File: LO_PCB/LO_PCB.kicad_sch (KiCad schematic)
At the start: 97 parts, among them J1 PWR, J2 Conn_01x06, Q1 AO3401A, U1 TPS7A9101DSKT, U2 LMX2582RHAR, X1 TB612-100.0M

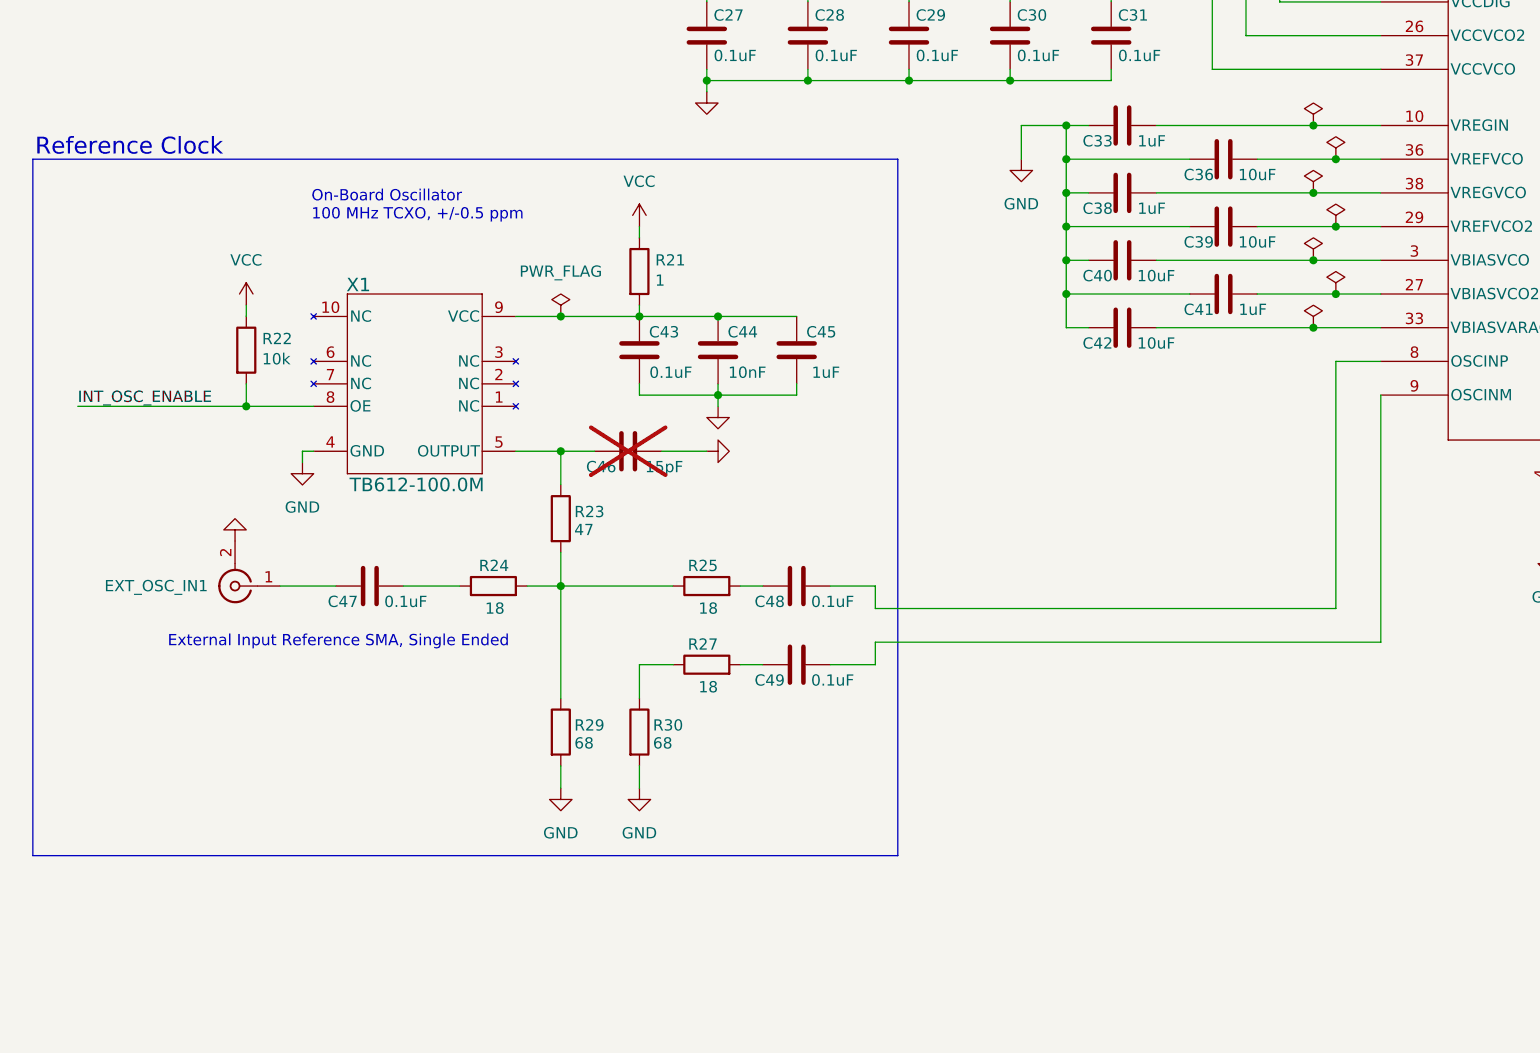
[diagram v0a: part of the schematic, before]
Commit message: final final LO PCB?
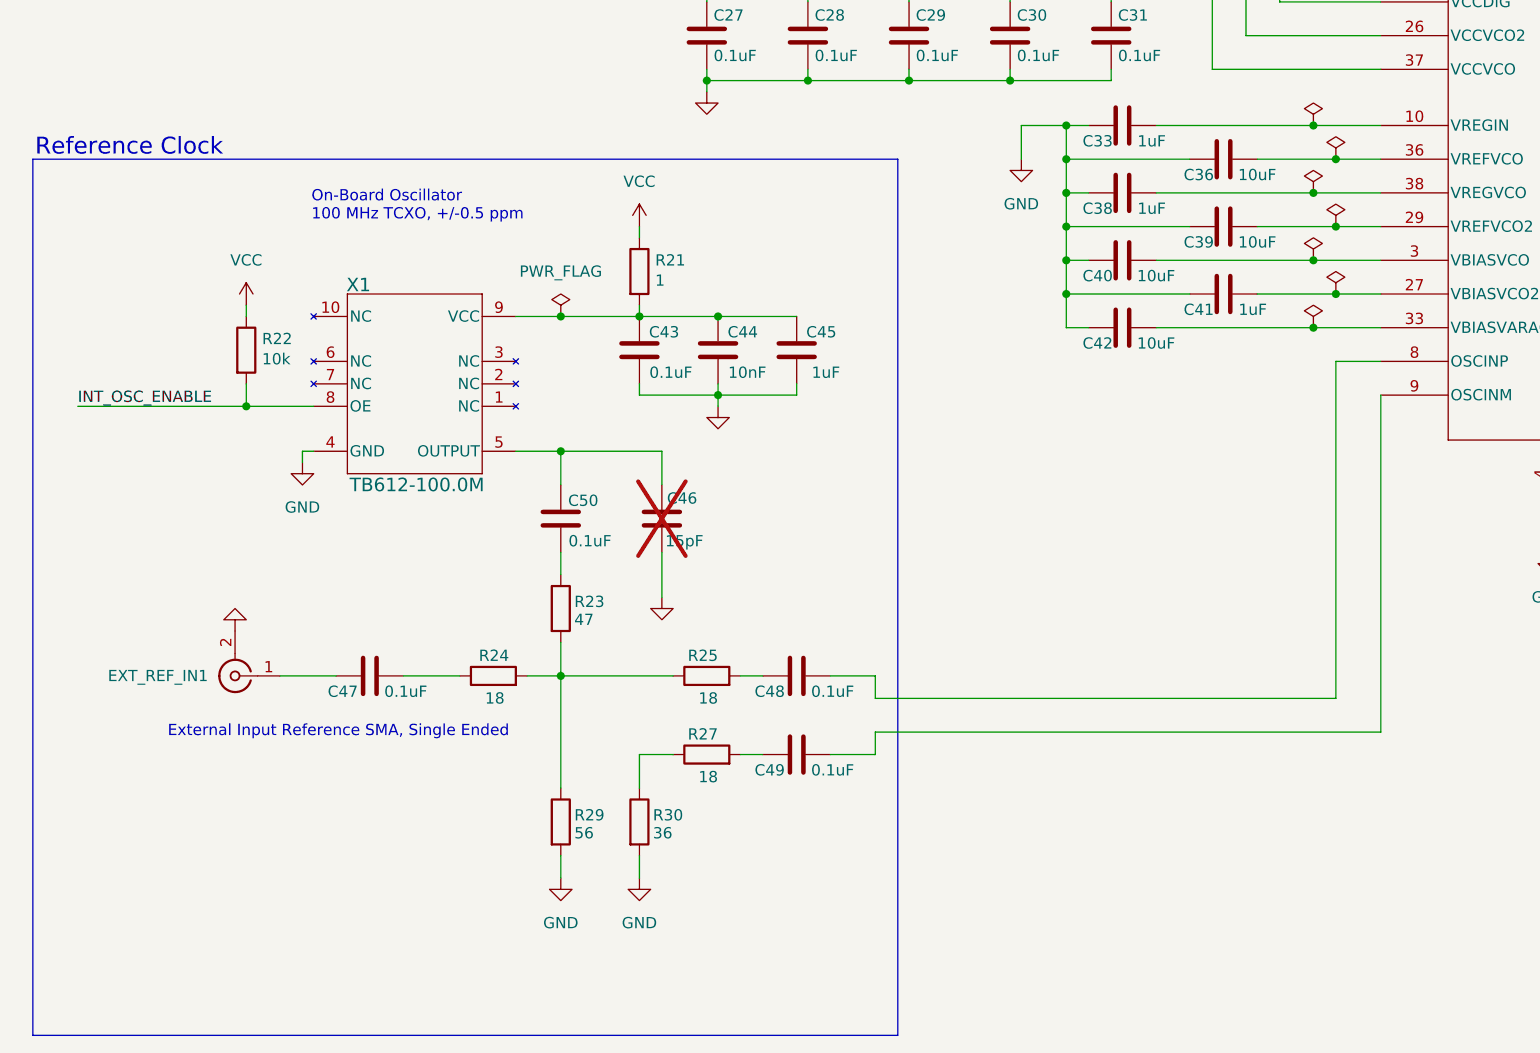
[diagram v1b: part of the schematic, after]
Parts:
- added C50: 0.1uF, Capacitor_SMD:C_0402_1005Metric, symbol Device:C
- C14, C16, C2, C23, C25, C36, C39, C4, C40, C42: Tolerance +/-20% -> +/-10%
- C44: MPN (none) -> GRM188R71H103KA01D; Manufacturer (none) -> Murata; Tolerance (none) -> +/-10%; Voltage (none) -> 50V
- C45: Dielectric X5R -> X7R; MPN (none) -> GRM188R71C105KA12D; Manufacturer (none) -> Murata; Tolerance (none) -> +/-10%; Voltage (none) -> 16V
- EXT_REF_IN1: renamed from EXT_OSC_IN1; value OSCinP -> EXT_REF_IN
- R1, R10, R11, R12, R13, R3: Tolerance +/-1% -> +/-0.1%
- R14, R15, R17, R18: Tolerance (none) -> +/-0.1%
- R19, R2, R21, R22, R26: Tolerance +/-5% -> +/-1%
- R20: Tolerance +/-1% -> +/-5%
- R23, R24, R25, R27: Tolerance +/-5% -> +/-0.1%
- R29: value 68 -> 56; MPN RG1005P-680-B-T5 -> RG1005P-560-B-T5; Tolerance +/-5% -> +/-0.1%
- R30: value 68 -> 36; MPN RG1005P-680-B-T5 -> RG1005P-360-B-T5; Tolerance +/-5% -> +/-0.1%
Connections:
- net at C46.1, X1.5 (OUTPUT): now also C50.2; no longer R23.1
- new net: C50.1, R23.1
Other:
- moved on the sheet: C46, C47, C48, C49, EXT_REF_IN1, R23, R24, R25, R27, R29, R30

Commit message: MPNs and some small stuff
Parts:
- C1, C13, C15, C22, C24, C43, C5: MPN GRM188R71H104KA93D -> GRM188R72A104KA35D
- C11, C33, C38, C41, C45: MPN GRM188R71C105KA12D -> 885012206052; Manufacturer Murata -> Würth Elektronik
- C14, C16, C2, C23, C25, C36, C39, C4, C40, C42: MPN GRM188R61A106KAALD -> GRT188R61A106KE13D
- C44: MPN GRM188R71H103KA01D -> GRM188R72A103KA01D
- R24, R25, R27: MPN RG1005P-180-B-T5 -> RC0402FR-0718RL; Manufacturer Susumu -> Yageo; Tolerance +/-0.1% -> +/-1%
- R30: MPN RG1005P-360-B-T5 -> ESR01MZPF36R0; Manufacturer Susumu -> Rohm; Tolerance +/-0.1% -> +/-1%
- X1: MPN (none) -> TB612-100.0M; Manufacturer (none) -> Connor-Winfield
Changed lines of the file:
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@@
 			)
 		)
-		(property "MPN" "GRM188R61A106KAALD"
+		(property "MPN" "GRT188R61A106KE13D"
 			(at 74.93 96.52 0)
 			(hide yes)
@@
 			)
 		)
-		(property "MPN" "RG1005P-360-B-T5"
+		(property "MPN" "ESR01MZPF36R0"
 			(at 106.68 227.33 0)
 			(hide yes)
@@
 			)
 		)
-		(property "Manufacturer" "Susumu"
+		(property "Manufacturer" "Rohm"
 			(at 106.68 227.33 0)
 			(hide yes)
@@
 			)
 		)
-		(property "Tolerance" "+/-0.1%"
+		(property "Tolerance" "+/-1%"
 			(at 106.68 227.33 0)
 			(hide yes)
@@
 			)
 		)
-		(property "MPN" "GRM188R71H104KA93D"
+		(property "MPN" "GRM188R72A104KA35D"
 			(at 64.77 115.57 0)
 			(hide yes)
@@
 			)
 		)
-		(property "MPN" "GRM188R71H104KA93D"
+		(property "MPN" "GRM188R72A104KA35D"
 			(at 85.09 115.57 0)
 			(hide yes)
@@
 			)
 		)
-		(property "MPN" "GRM188R71C105KA12D"
+		(property "MPN" "885012206052"
 			(at 161.29 148.59 0)
 			(hide yes)
@@
 			)
 		)
-		(property "Manufacturer" "Murata"
+		(property "Manufacturer" "Würth Elektronik"
 			(at 161.29 148.59 0)
 			(hide yes)
@@
 			)
 		)
-		(property "MPN" "GRM188R61A106KAALD"
+		(property "MPN" "GRT188R61A106KE13D"
 			(at 161.29 163.83 0)
 			(hide yes)
@@
 			)
 		)
-		(property "MPN" "GRM188R61A106KAALD"
+		(property "MPN" "GRT188R61A106KE13D"
 			(at 95.25 115.57 0)
 			(hide yes)
@@
 			)
 		)
-		(property "MPN" "GRM188R71H104KA93D"
+		(property "MPN" "GRM188R72A104KA35D"
 			(at 167.64 55.88 0)
 			(hide yes)
@@
 			)
 		)
-		(property "MPN" "GRM188R71C105KA12D"
+		(property "MPN" "885012206052"
 			(at 124.46 173.99 0)
 			(hide yes)
@@
 			)
 		)
-		(property "Manufacturer" "Murata"
+		(property "Manufacturer" "Würth Elektronik"
 			(at 124.46 173.99 0)
 			(hide yes)
@@
 			)
 		)
-		(property "MPN" "GRM188R61A106KAALD"
+		(property "MPN" "GRT188R61A106KE13D"
 			(at 95.25 96.52 0)
 			(hide yes)
@@
 			)
 		)
-		(property "MPN" "GRM188R71H104KA93D"
+		(property "MPN" "GRM188R72A104KA35D"
 			(at 106.68 173.99 0)
 			(hide yes)
@@
 			)
 		)
-		(property "MPN" "GRM188R61A106KAALD"
+		(property "MPN" "GRT188R61A106KE13D"
 			(at 160.02 55.88 0)
 			(hide yes)
@@
 			)
 		)
-		(property "MPN" "GRM188R61A106KAALD"
+		(property "MPN" "GRT188R61A106KE13D"
 			(at 92.71 55.88 0)
 			(hide yes)
@@
 			)
 		)
-		(property "MPN" "GRM188R61A106KAALD"
+		(property "MPN" "GRT188R61A106KE13D"
 			(at 172.72 152.4 0)
 			(hide yes)
@@
 			)
 		)
-		(property "MPN" "RG1005P-180-B-T5"
+		(property "MPN" "RC0402FR-0718RL"
 			(at 90.17 210.82 0)
 			(hide yes)
@@
 			)
 		)
-		(property "Manufacturer" "Susumu"
+		(property "Manufacturer" "Yageo"
 			(at 90.17 210.82 0)
 			(hide yes)
@@
 			)
 		)
-		(property "Tolerance" "+/-0.1%"
+		(property "Tolerance" "+/-1%"
 			(at 90.17 210.82 0)
 			(hide yes)
@@
 			)
 		)
+		(property "MPN" "TB612-100.0M"
+			(at 81.28 165.1 0)
+			(hide yes)
+			(show_name no)
+			(do_not_autoplace no)
+			(effects
+				(font
+					(size 1.27 1.27)
+				)
+			)
+		)
+		(property "Manufacturer" "Connor-Winfield"
+			(at 81.28 165.1 0)
+			(hide yes)
+			(show_name no)
+			(do_not_autoplace no)
+			(effects
+				(font
+					(size 1.27 1.27)
+				)
+			)
+		)
 		(pin "10"
 		)
@@
 			)
 		)
-		(property "MPN" "GRM188R61A106KAALD"
+		(property "MPN" "GRT188R61A106KE13D"
 			(at 161.29 171.45 0)
 			(hide yes)
@@
 			)
 		)
-		(property "MPN" "GRM188R71C105KA12D"
+		(property "MPN" "885012206052"
 			(at 172.72 167.64 0)
 			(hide yes)
@@
 			)
 		)
-		(property "Manufacturer" "Murata"
+		(property "Manufacturer" "Würth Elektronik"
 			(at 172.72 167.64 0)
 			(hide yes)
@@
 			)
 		)
-		(property "MPN" "GRM188R71C105KA12D"
+		(property "MPN" "885012206052"
 			(at 161.29 156.21 0)
 			(hide yes)
@@
 			)
 		)
-		(property "Manufacturer" "Murata"
+		(property "Manufacturer" "Würth Elektronik"
 			(at 161.29 156.21 0)
 			(hide yes)
@@
 			)
 		)
-		(property "MPN" "GRM188R61A106KAALD"
+		(property "MPN" "GRT188R61A106KE13D"
 			(at 74.93 115.57 0)
 			(hide yes)
@@
 			)
 		)
-		(property "MPN" "GRM188R71H104KA93D"
+		(property "MPN" "GRM188R72A104KA35D"
 			(at 85.09 96.52 0)
 			(hide yes)
@@
 			)
 		)
-		(property "MPN" "GRM188R71H103KA01D"
+		(property "MPN" "GRM188R72A103KA01D"
 			(at 115.57 173.99 0)
 			(hide yes)
@@
 			)
 		)
-		(property "MPN" "GRM188R71C105KA12D"
+		(property "MPN" "885012206052"
 			(at 101.6 71.12 0)
 			(hide yes)
@@
 			)
 		)
-		(property "Manufacturer" "Murata"
+		(property "Manufacturer" "Würth Elektronik"
 			(at 101.6 71.12 0)
 			(hide yes)
@@
 			)
 		)
-		(property "MPN" "GRM188R61A106KAALD"
+		(property "MPN" "GRT188R61A106KE13D"
 			(at 172.72 160.02 0)
 			(hide yes)
@@
 			)
 		)
-		(property "MPN" "RG1005P-180-B-T5"
+		(property "MPN" "RC0402FR-0718RL"
 			(at 114.3 210.82 0)
 			(hide yes)
@@
 			)
 		)
-		(property "Manufacturer" "Susumu"
+		(property "Manufacturer" "Yageo"
 			(at 114.3 210.82 0)
 			(hide yes)
@@
 			)
 		)
-		(property "Tolerance" "+/-0.1%"
+		(property "Tolerance" "+/-1%"
 			(at 114.3 210.82 0)
 			(hide yes)
@@
 			)
 		)
-		(property "MPN" "GRM188R71H104KA93D"
+		(property "MPN" "GRM188R72A104KA35D"
 			(at 85.09 55.88 0)
 			(hide yes)
@@
 			)
 		)
-		(property "MPN" "GRM188R71H104KA93D"
+		(property "MPN" "GRM188R72A104KA35D"
 			(at 64.77 96.52 0)
 			(hide yes)
@@
 			)
 		)
-		(property "MPN" "RG1005P-180-B-T5"
+		(property "MPN" "RC0402FR-0718RL"
 			(at 114.3 219.71 0)
 			(hide yes)
@@
 			)
 		)
-		(property "Manufacturer" "Susumu"
+		(property "Manufacturer" "Yageo"
 			(at 114.3 219.71 0)
 			(hide yes)
@@
 			)
 		)
-		(property "Tolerance" "+/-0.1%"
+		(property "Tolerance" "+/-1%"
 			(at 114.3 219.71 0)
 			(hide yes)
